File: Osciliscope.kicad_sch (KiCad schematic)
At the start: 69 parts, among them J1 Conn_01x09_Socket, J2 Conn_01x04_Socket, J3 U.FL, J4 Conn_01x04_Socket, J5 USB_C_Receptacle_USB2.0_14P, J6 Conn_01x02_MountingPin, J7 U.FL, J8 USB_C_Receptacle_USB2.0_14P, J9 Conn_01x03_Socket, SW1 RotaryEncoder_Switch, SW2 SW_SPST, SW4 SW_Nidec_CAS-120A1, SW5 RotaryEncoder_Switch, SW6 RotaryEncoder_Switch, SW7 SW_Nidec_CAS-120A1, U1 MCP1700x-330xxMB, U2 ADC082S101, U3 CH340N, U5 TLV9061xDBV, U6 TLV9061xDBV, U7 TLV9061xDBV

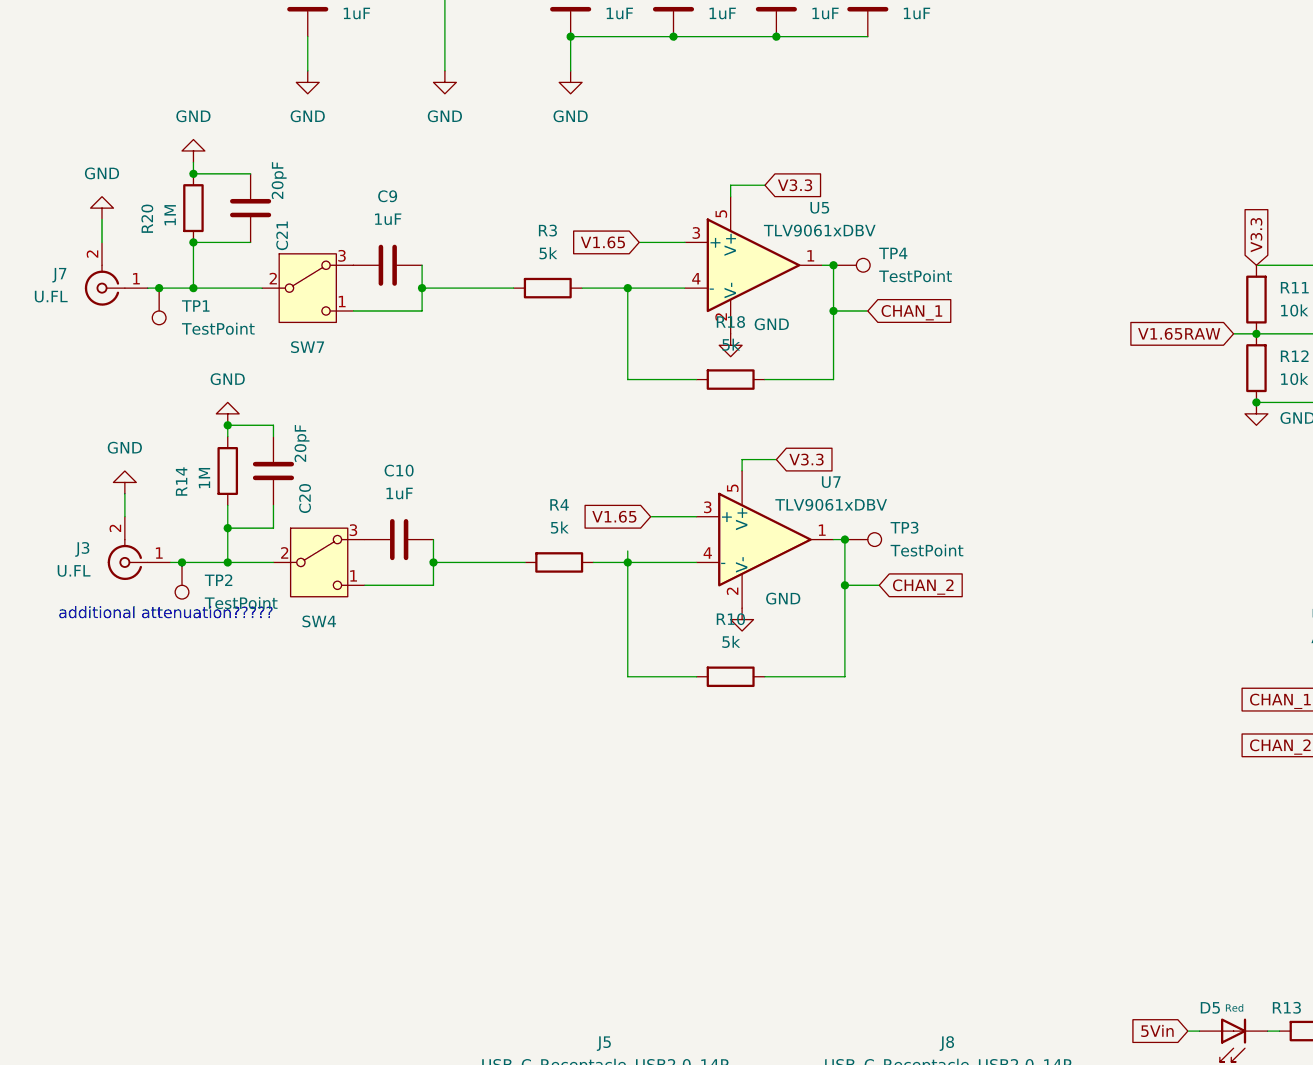
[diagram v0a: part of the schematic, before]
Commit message: changes to lots of stuff
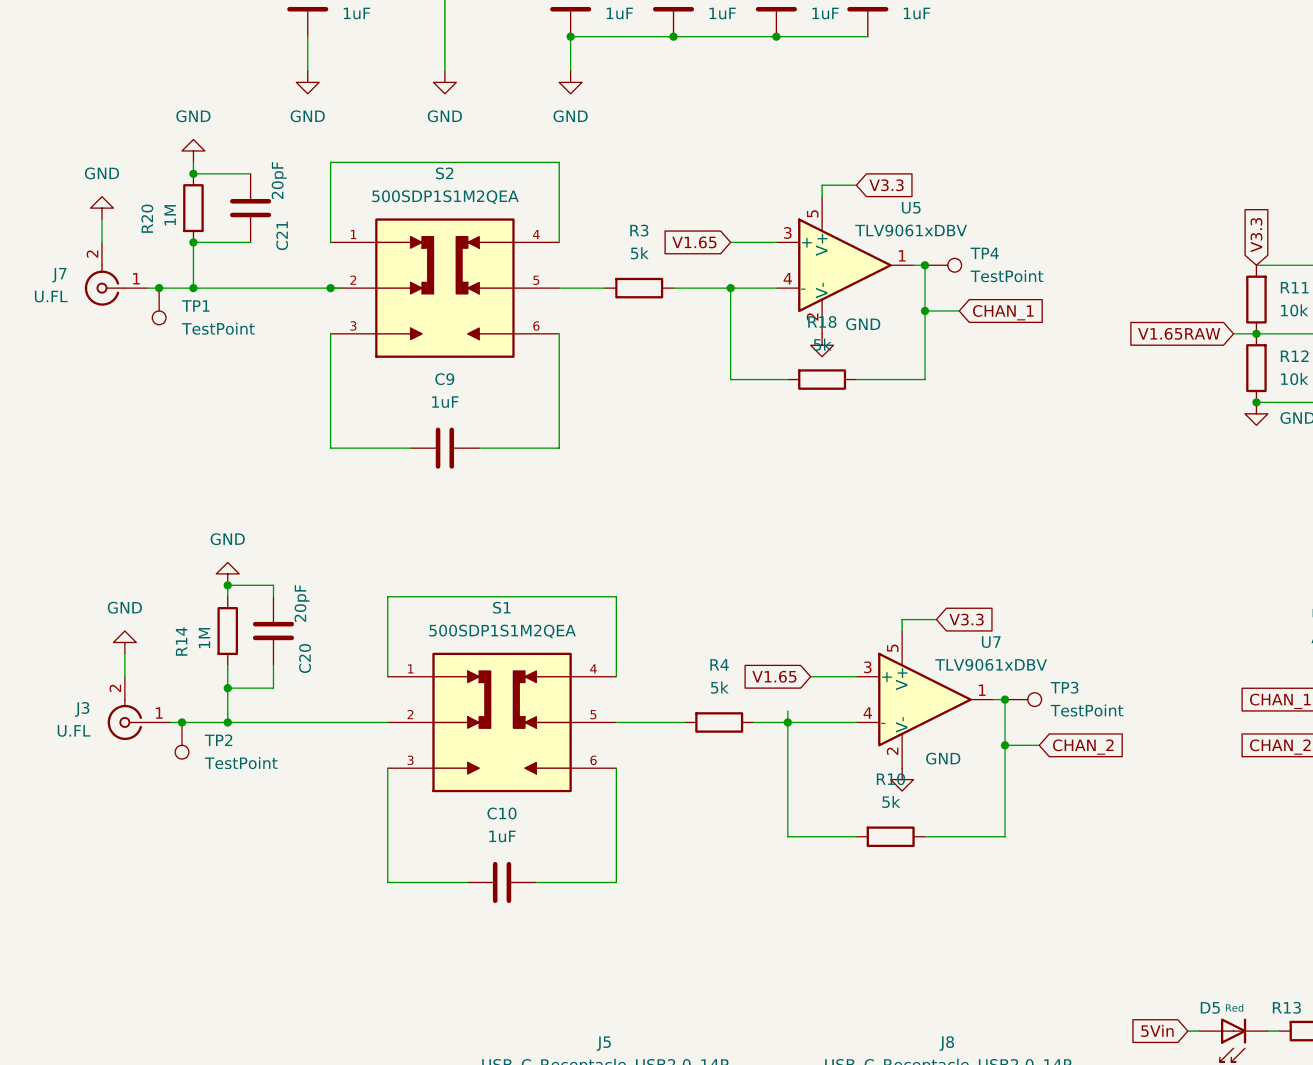
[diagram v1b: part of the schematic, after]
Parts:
- removed SW4, SW7: SW_Nidec_CAS-120A1, Button_Switch_SMD:Nidec_Copal_CAS-120A, symbol Switch:SW_Nidec_CAS-120A1
- added S1, S2: 500SDP1S1M2QEA, 500SDP1S1M2QEA:SW_500SDP1S1M2QEA, symbol 500SDP1S1M2QEA:500SDP1S1M2QEA
- C10, C9: footprint Capacitor_SMD:C_1206_3216Metric -> (none)
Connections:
- net at C21.2, J7.1 (In), R20.2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: now also S2.2
- net at C20.2, J3.1 (In), R14.2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: now also S1.2
- net at R3.2: now also S2.5; no longer C9.2
- net at C9.1: now also S2.3
- net at C10.1: now also S1.3
- net at R4.2: now also S1.5; no longer C10.2
- new net: S2.1, S2.4
- new net: C9.2, S2.6
- new net: S1.1, S1.4
- new net: C10.2, S1.6
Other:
- note removed: "additional attenuation?????"
- moved on the sheet: C20, J3, R10, R14, R18, R3, R4, TP2, TP3, TP4, U5, U7
